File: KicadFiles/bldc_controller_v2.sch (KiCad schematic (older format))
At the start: 184 parts, among them J1 Conn_01x06_Male, J10 Conn_01x02_Female, J11 Conn_01x02_Female, J12 Conn_01x02_Female, J13 Conn_01x02_Female, J14 Conn_01x02_Female, J15 Conn_01x04_Male, J2 Conn_01x03_Male, J3 Conn_01x03_Male, J4 Screw_Terminal, J5 Conn_01x02_Female, J9 Conn_01x02_Female, Q1 DMN65D8L-7, Q10 IRLB8721PBF, Q11 IRLB8721PBF, Q2 DMN65D8L-7, Q3 DMN65D8L-7, Q4 DMN65D8L-7, Q5 IRF4905, Q6 IRLB8721PBF, Q7 IRLB8721PBF, Q8 IRLB8721PBF, Q9 IRLB8721PBF, SW1 D6C50 F1 LFS, SW2 D6C40 F1 LFS, SW3 1301.9314, SW4 1301.9314, SW5 SW_Push_DPDT, U1 ATmega328P-PU, U2 uA7810, U3 LM7805_TO220, U4 MCP601-xP, U5 LM339, U6 IRS2004, U7 IRS2004, U8 IRS2004, Y1 9B-16.000MBBK-B

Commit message: Ready for Parts Placement
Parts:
- C1, C19, C2, C7: footprint Capacitor_THT:CP_Radial_D10.0mm_P5.00mm -> Capacitor_THT:CP_Radial_D5.0mm_P2.00mm
- J10, J11, J12, J13, J14, J5, J9: footprint (none) -> Connector_PinHeader_2.54mm:PinHeader_1x02_P2.54mm_Vertical
- J15: footprint (none) -> Connector_PinHeader_2.54mm:PinHeader_1x04_P2.54mm_Vertical
- J2, J3: footprint (none) -> Connector_PinHeader_2.54mm:PinHeader_1x03_P2.54mm_Vertical
- SW3: footprint Button_Switch_THT:Pushbutton_Switch_TH -> Button_Switch_SMD:Tactile_Switch_SM
- SW5: footprint (none) -> Button_Switch_SMD:Slide_Switch_DPDT_SMD
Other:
- moved on the sheet: C1, C10, C11, C12, C13, C14, C15, C16, C17, C18, C19, C2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

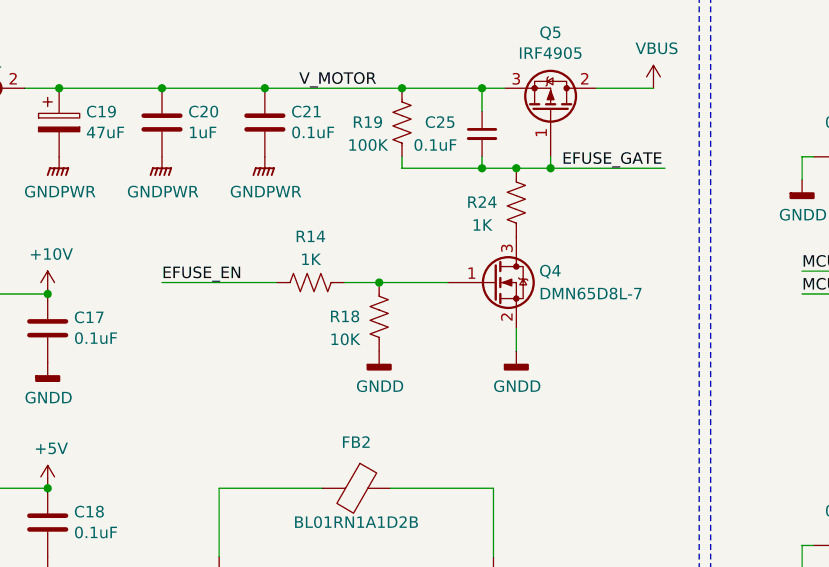
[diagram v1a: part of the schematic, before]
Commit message: Cleaned Up Repo
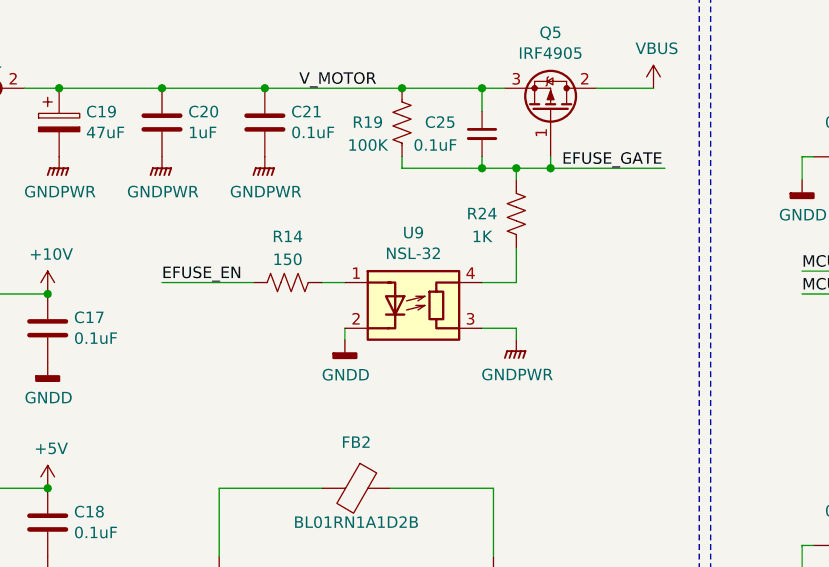
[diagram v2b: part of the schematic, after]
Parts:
- removed Q4: DMN65D8L-7, Package_TO_SOT_SMD:SOT-23, symbol Transistor_FET:DMN67D7L
- removed R18: 10K, Resistor_SMD:R_0805_2012Metric_Pad1.15x1.40mm_HandSolder, symbol Device:R_US
- added U9: NSL-32, symbol Isolator:NSL-32
- R14: value 1K -> 150
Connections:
- wire segments 336 -> 340
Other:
- moved on the sheet: R14, R24
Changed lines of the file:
@@
 L Device:R_US R24
 U 1 1 5E18B694
-P 9100 1500
-F 0 "R24" H 8950 1500 50  0000 C CNN
-F 1 "1K" H 8950 1400 50  0000 C CNN
-F 2 "Resistor_SMD:R_0805_2012Metric_Pad1.15x1.40mm_HandSolder" V 9140 1490 50  0001 C CNN
-F 3 "~" H 9100 1500 50  0001 C CNN
-	1    9100 1500
+P 9100 1550
+F 0 "R24" H 8950 1550 50  0000 C CNN
+F 1 "1K" H 8950 1450 50  0000 C CNN
+F 2 "Resistor_SMD:R_0805_2012Metric_Pad1.15x1.40mm_HandSolder" V 9140 1540 50  0001 C CNN
+F 3 "~" H 9100 1550 50  0001 C CNN
+	1    9100 1550
 	1    0    0    -1
 $EndComp
@@
 L Device:R_US R14
 U 1 1 5E1991B6
-P 8200 1850
-F 0 "R14" V 8000 1850 50  0000 C CNN
-F 1 "1K" V 8100 1850 50  0000 C CNN
-F 2 "Resistor_SMD:R_0805_2012Metric_Pad1.15x1.40mm_HandSolder" V 8240 1840 50  0001 C CNN
-F 3 "~" H 8200 1850 50  0001 C CNN
-	1    8200 1850
+P 8100 1850
+F 0 "R14" V 7900 1850 50  0000 C CNN
+F 1 "150" V 8000 1850 50  0000 C CNN
+F 2 "Resistor_SMD:R_0805_2012Metric_Pad1.15x1.40mm_HandSolder" V 8140 1840 50  0001 C CNN
+F 3 "~" H 8100 1850 50  0001 C CNN
+	1    8100 1850
 	0    1    1    0
 $EndComp
 Text Label 7550 1850 0    50   ~ 0
 EFUSE_EN
-$Comp
-L Device:R_US R18
-U 1 1 5E0E4EED
-P 8500 2000
-F 0 "R18" H 8350 2000 50  0000 C CNN
-F 1 "10K" H 8350 1900 50  0000 C CNN
-F 2 "Resistor_SMD:R_0805_2012Metric_Pad1.15x1.40mm_HandSolder" V 8540 1990 50  0001 C CNN
-F 3 "~" H 8500 2000 50  0001 C CNN
-	1    8500 2000
-	1    0    0    -1
-$EndComp
-$Comp
-L power:GNDD #PWR084
-U 1 1 5E62DD30
-P 9100 2150
-F 0 "#PWR084" H 9100 1900 50  0001 C CNN
-F 1 "GNDD" H 9104 1995 50  0000 C CNN
-F 2 "" H 9100 2150 50  0001 C CNN
-F 3 "" H 9100 2150 50  0001 C CNN
-	1    9100 2150
-	1    0    0    -1
-$EndComp
 Connection ~ 8600 1000
 $Comp
@@
 Wire Wire Line
 	8550 2750 9000 2750
-$Comp
-L Transistor_FET:DMN67D7L Q4
-U 1 1 5E2655F0
-P 9000 1850
-F 0 "Q4" H 9200 1900 50  0000 L CNN
-F 1 "DMN65D8L-7" H 9200 1800 50  0000 L CNN
-F 2 "Package_TO_SOT_SMD:SOT-23" H 9200 1775 50  0001 L CIN
-F 3 "http://www.diodes.com/assets/Datasheets/DMN67D7L.pdf" H 9000 1850 50  0001 L CNN
-	1    9000 1850
-	1    0    0    -1
-$EndComp
-Wire Wire Line
-	8350 1850 8500 1850
 Text Label 8150 1000 0    50   ~ 0
 V_MOTOR
@@
 	9250 1300 9250 1350
 Wire Wire Line
-	8800 1850 8500 1850
-Connection ~ 8500 1850
-Wire Wire Line
-	9100 2050 9100 2150
-$Comp
-L power:GNDD #PWR077
-U 1 1 5FBEC279
-P 8500 2150
-F 0 "#PWR077" H 8500 1900 50  0001 C CNN
-F 1 "GNDD" H 8504 1995 50  0000 C CNN
-F 2 "" H 8500 2150 50  0001 C CNN
-F 3 "" H 8500 2150 50  0001 C CNN
-	1    8500 2150
-	1    0    0    -1
-$EndComp
-Wire Wire Line
 	8000 1000 8600 1000
 $Comp
@@
 Wire Wire Line
 	8600 1350 8950 1350
-Connection ~ 9250 1350
-Connection ~ 9100 1350
-Wire Wire Line
-	9100 1350 9250 1350
 Wire Wire Line
 	8950 1300 8950 1350
-Connection ~ 8950 1350
-Wire Wire Line
-	8950 1350 9100 1350
 Wire Wire Line
 	8950 1100 8950 1000
@@
 $EndComp
 Wire Wire Line
-	7550 1850 8050 1850
+	7550 1850 7950 1850
 Wire Wire Line
 	7800 2750 8250 2750
@@
 NoConn ~ 7050 6500
 NoConn ~ 7050 6700
+$Comp
+L power:GNDPWR #PWR084
+U 1 1 5E09A255
+P 9100 2100
+F 0 "#PWR084" H 9100 1900 50  0001 C CNN
+F 1 "GNDPWR" H 9104 1946 50  0000 C CNN
+F 2 "" H 9100 2050 50  0001 C CNN
+F 3 "" H 9100 2050 50  0001 C CNN
+	1    9100 2100
+	1    0    0    -1
+$EndComp
+Wire Wire Line
+	9100 2050 9100 2100
+$Comp
+L Isolator:NSL-32 U9
+U 1 1 5E0D9513
+P 8650 1950
+F 0 "U9" H 8650 2267 50  0000 C CNN
+F 1 "NSL-32" H 8650 2176 50  0000 C CNN
+F 2 "" H 8650 1650 50  0001 C CNN
+F 3 "http://lunainc.com/wp-content/uploads/2016/06/NSL-32.pdf" H 8700 1950 50  0001 C CNN
+	1    8650 1950
+	1    0    0    -1
+$EndComp
+Wire Wire Line
+	8350 1850 8250 1850
+$Comp
+L power:GNDD #PWR077
+U 1 1 5E17C602
+P 8350 2100
+F 0 "#PWR077" H 8350 1850 50  0001 C CNN
+F 1 "GNDD" H 8354 1945 50  0000 C CNN
+F 2 "" H 8350 2100 50  0001 C CNN
+F 3 "" H 8350 2100 50  0001 C CNN
+	1    8350 2100
+	1    0    0    -1
+$EndComp
+Wire Wire Line
+	8350 2050 8350 2100
+Wire Wire Line
+	8950 2050 9100 2050
+Wire Wire Line
+	8950 1850 9100 1850
+Wire Wire Line
+	9100 1850 9100 1700
+Wire Wire Line
+	8950 1350 9100 1350
+Connection ~ 8950 1350
+Connection ~ 9250 1350
+Wire Wire Line
+	9100 1350 9100 1400
+Connection ~ 9100 1350
+Wire Wire Line
+	9100 1350 9250 1350
 $EndSCHEMATC
